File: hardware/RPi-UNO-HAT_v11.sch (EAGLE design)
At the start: 61 parts, among them IC1 24LC-I/OT, IC2 ATMEGA328-AU, IC3 LDO-TS9011-3V3, Q1 16MHz, T1 BSS138PS, T2 BSS138PS, T3 BSS138PS, X1 PASSER-07, X2 PASSER-07, X3 PASSER-07

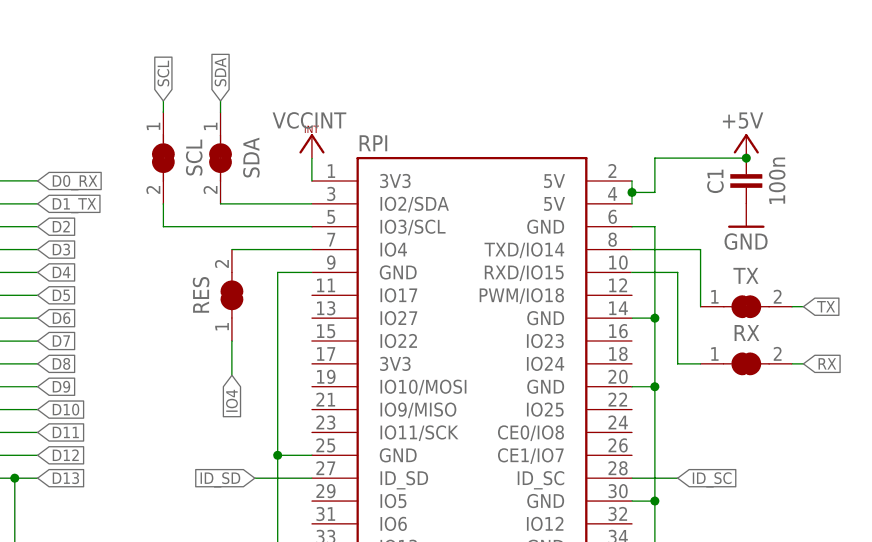
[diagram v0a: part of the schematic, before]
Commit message: updated layout and schematics
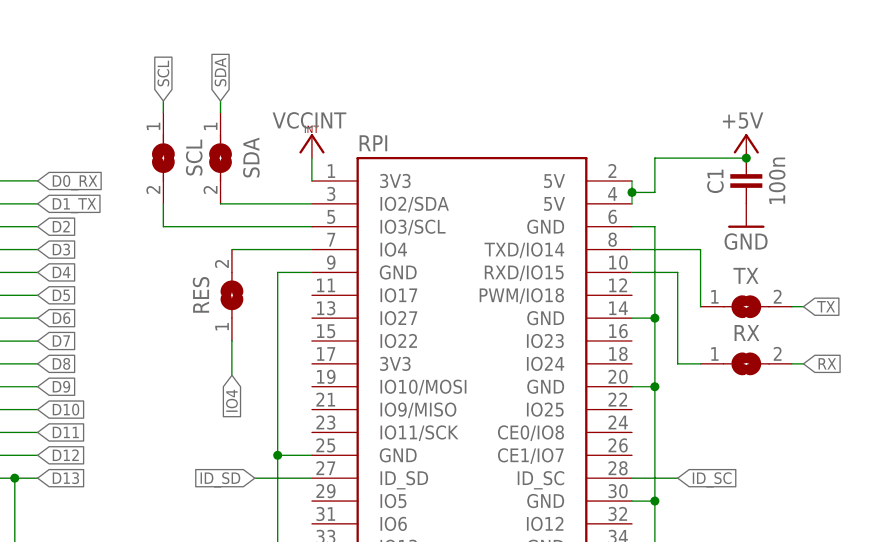
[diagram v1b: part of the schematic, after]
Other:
- note removed: "Note/Bug: D0/Rx is not connected to pin 4 TXO"
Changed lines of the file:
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@@
 <text x="62.23" y="27.94" size="3.81" layer="250">Power Supply</text>
 <text x="199.39" y="92.71" size="3.81" layer="250">external FTDI</text>
-<text x="234.95" y="76.2" size="1.778" layer="250">Note/Bug:
-D0/Rx is not
-connected
-to pin 4 TXO</text>
-<wire x1="180.34" y1="160.655" x2="180.34" y2="159.385" width="0.3048" layer="94"/>
-<wire x1="186.69" y1="160.655" x2="186.69" y2="159.385" width="0.3048" layer="94"/>
-<wire x1="187.96" y1="145.415" x2="187.96" y2="144.145" width="0.3048" layer="94"/>
-<wire x1="244.475" y1="143.51" x2="245.745" y2="143.51" width="0.3048" layer="94"/>
-<wire x1="244.475" y1="137.16" x2="245.745" y2="137.16" width="0.3048" layer="94"/>
 </plain>
 <instances>
